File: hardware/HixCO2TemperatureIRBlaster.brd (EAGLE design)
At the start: 119.4 x 94 mm, 36 parts, among them J1 FTDI, J2 IEC320C8, J3 XH4P, Q1 AO3400, Q2 AO3400, U1 TSOP2238, U2 LM3940, U3 HLK-PM01, U4 DS18B20

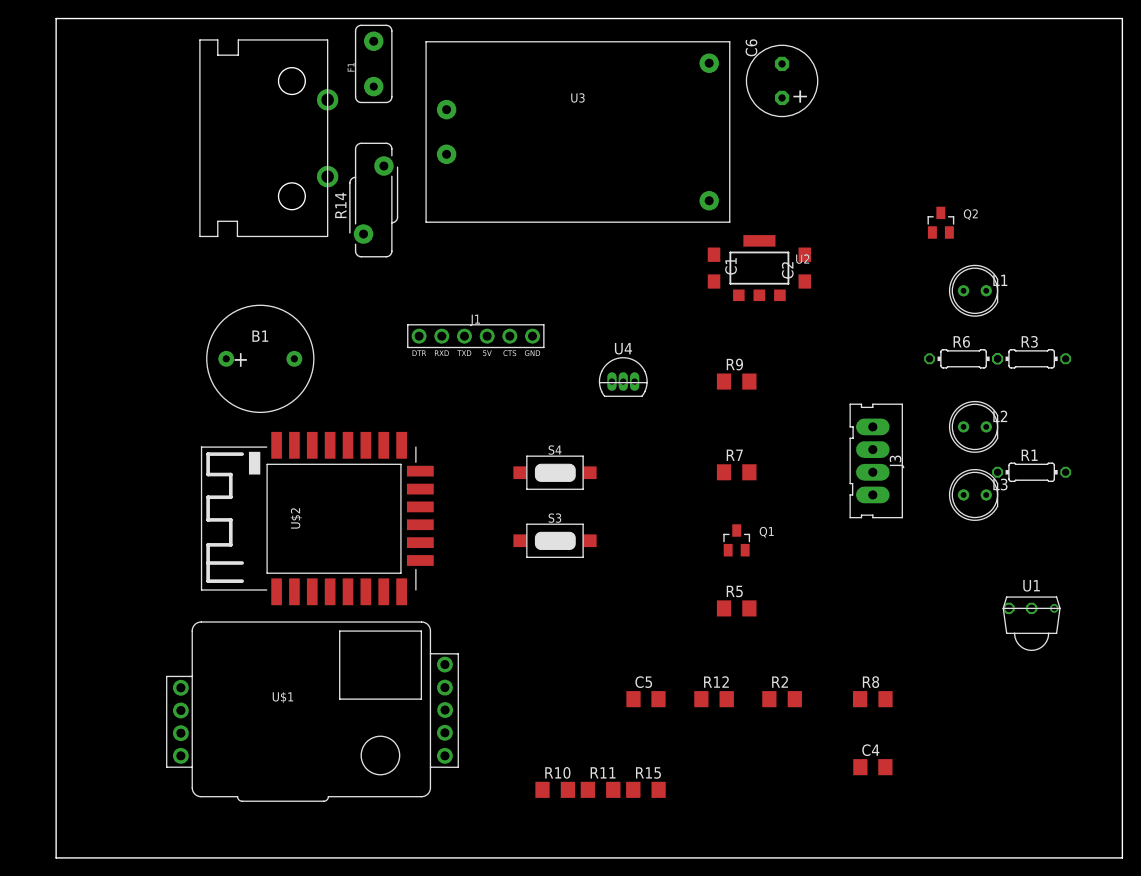
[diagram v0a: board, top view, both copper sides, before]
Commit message: electronic hardware v1 complete
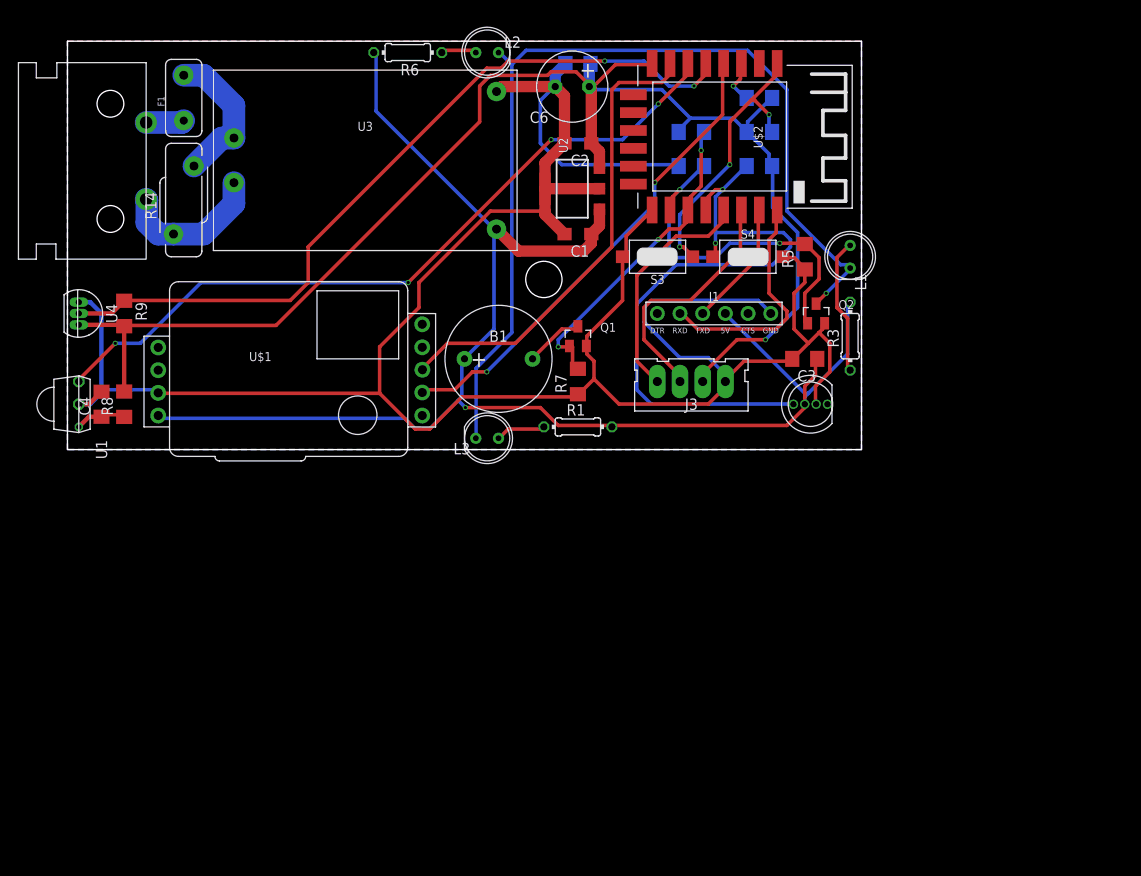
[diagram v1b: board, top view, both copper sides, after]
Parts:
- added C3: 100nF, rcl:C1206
- added U$3: LED_RGB, 0_HixField:LED_PL9823-F5
- F1: value 800mA -> 800mA 250V
- moved U1 108.2 mm to (-129.5, -264.2), turned to 270 degrees
- moved C4 95.4 mm to (-129.5, -261.6), turned to 90 degrees
- moved R8 90.1 mm to (-127.0, -261.6), turned to 90 degrees
- moved R11 79.5 mm to (-55.9, -227.3), flipped to the bottom, turned to 180 degrees
- moved R10 77.1 mm to (-55.9, -231.1), flipped to the bottom
- moved C5 71.5 mm to (-76.2, -223.5), flipped to the bottom
- moved R6 71.1 mm to (-95.2, -222.2), turned to 180 degrees
- moved R15 71.0 mm to (-55.9, -234.9), flipped to the bottom, turned to 180 degrees
- moved R9 69.0 mm to (-127.0, -251.5), turned to 270 degrees
- moved L2 68.8 mm to (-87.6, -222.2)
- moved R12 63.6 mm to (-63.5, -231.1), flipped to the bottom
- moved U$2 61.5 mm to (-59.7, -231.8), turned to 270 degrees
- moved U4 61.4 mm to (-132.1, -251.5), turned to 270 degrees
- moved R2 60.5 mm to (-63.5, -234.9), flipped to the bottom, turned to 180 degrees
- moved L3 52.5 mm to (-85.1, -265.4), turned to 180 degrees
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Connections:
- net 5.0V: now also C3.1, U$3.VCC
- net GND: now also C3.2, U$3.GND
- net RGB: now also U$3.DIN
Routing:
- net GND: track 0.00 -> 272.3 mm
- net 5.0V: track 0.00 -> 171.9 mm, vias 0 -> 1
- net 3.3V: track 0.00 -> 163.2 mm, vias 0 -> 1
- net N$3: track 0.00 -> 107.9 mm, vias 0 -> 1
- net TEMP: track 0.00 -> 87.1 mm, vias 0 -> 2
- net IR_IN: track 0.00 -> 83.7 mm, vias 0 -> 4
- net RGB: track 0.00 -> 72.4 mm, vias 0 -> 2
- net CO2_TX: track 0.00 -> 53.8 mm, vias 0 -> 2
- net CO2_RX: track 0.00 -> 53.0 mm
- net IR_OUT: track 0.00 -> 40.6 mm, vias 0 -> 2
- net BEEP: track 0.00 -> 36.1 mm, vias 0 -> 3
- net N$7: track 0.00 -> 31.7 mm, vias 0 -> 3
- net SCL: track 0.00 -> 28.3 mm
- net RXD: track 0.00 -> 26.5 mm
- net SDA: track 0.00 -> 26.3 mm
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- added copper zone on layer 16, net 3.3V
- added copper zone on layer 16, net 5.0V
- added copper zone on layer 1, net GND
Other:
- board size 119.4 x 94 mm -> 88.9 x 45.7 mm
